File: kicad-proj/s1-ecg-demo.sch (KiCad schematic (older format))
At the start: 56 parts, among them J1 USB-C-16-Pin, J2 TC2030, J3 Battery Port, J4 Current Probe, J5 ECG_PAD_LA, J6 ECG_PAD_RA, J7 ECG_PAD_RL, U1 AD8233

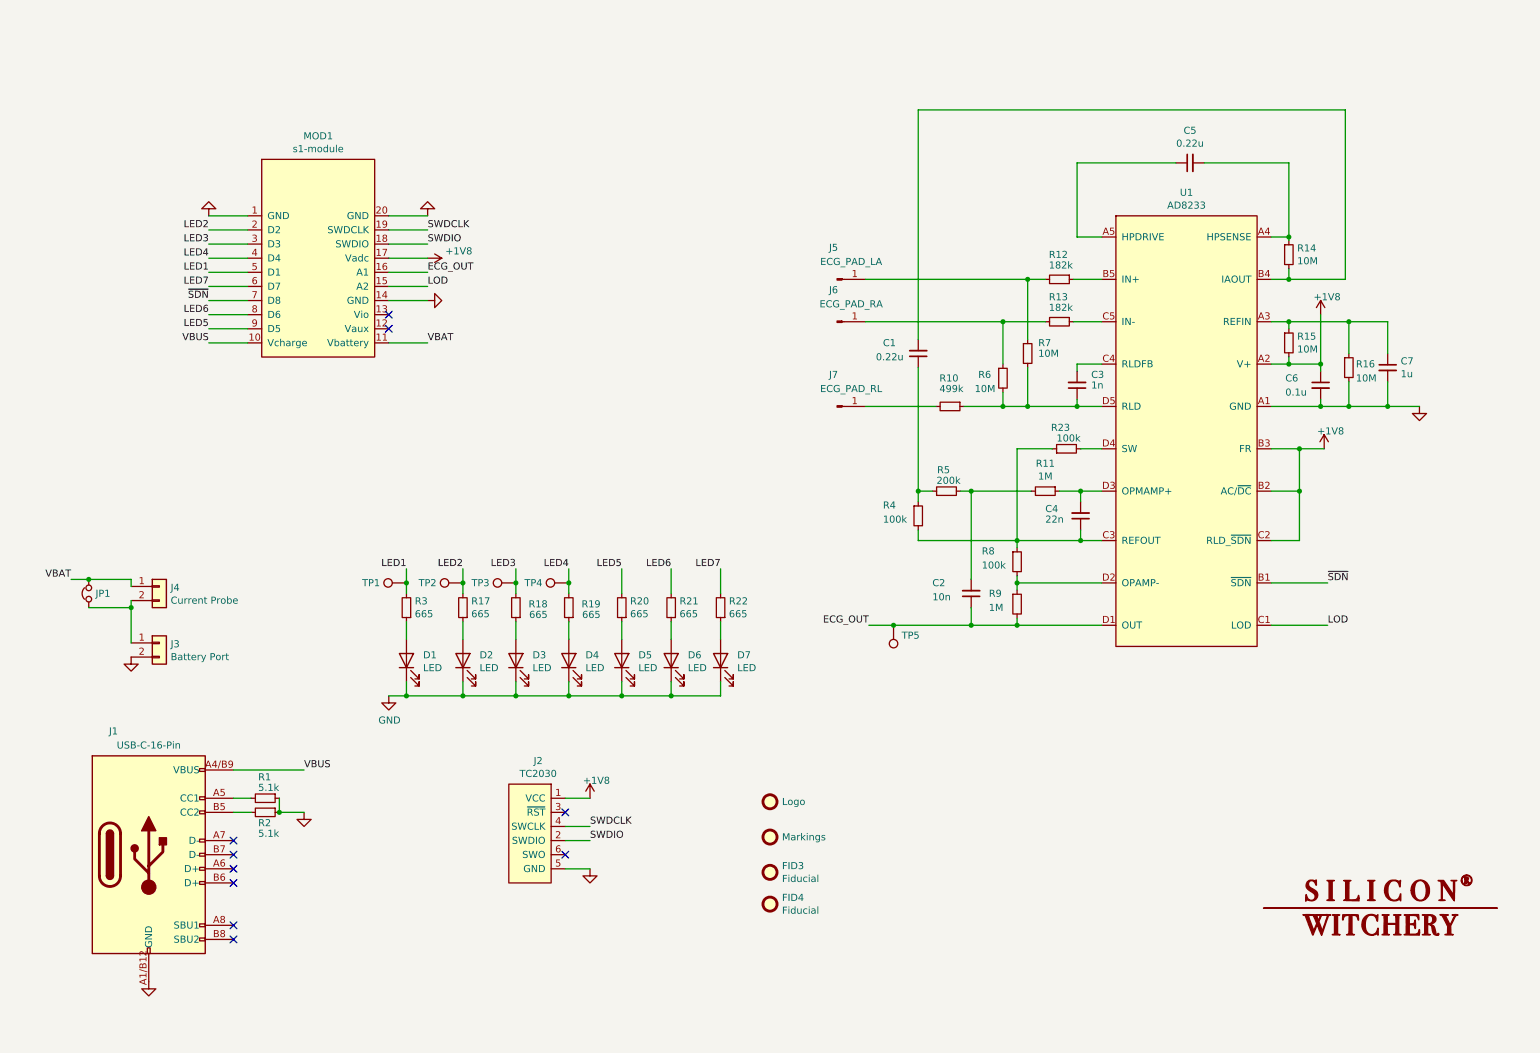
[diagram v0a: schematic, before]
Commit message: Layout complete, needs checking
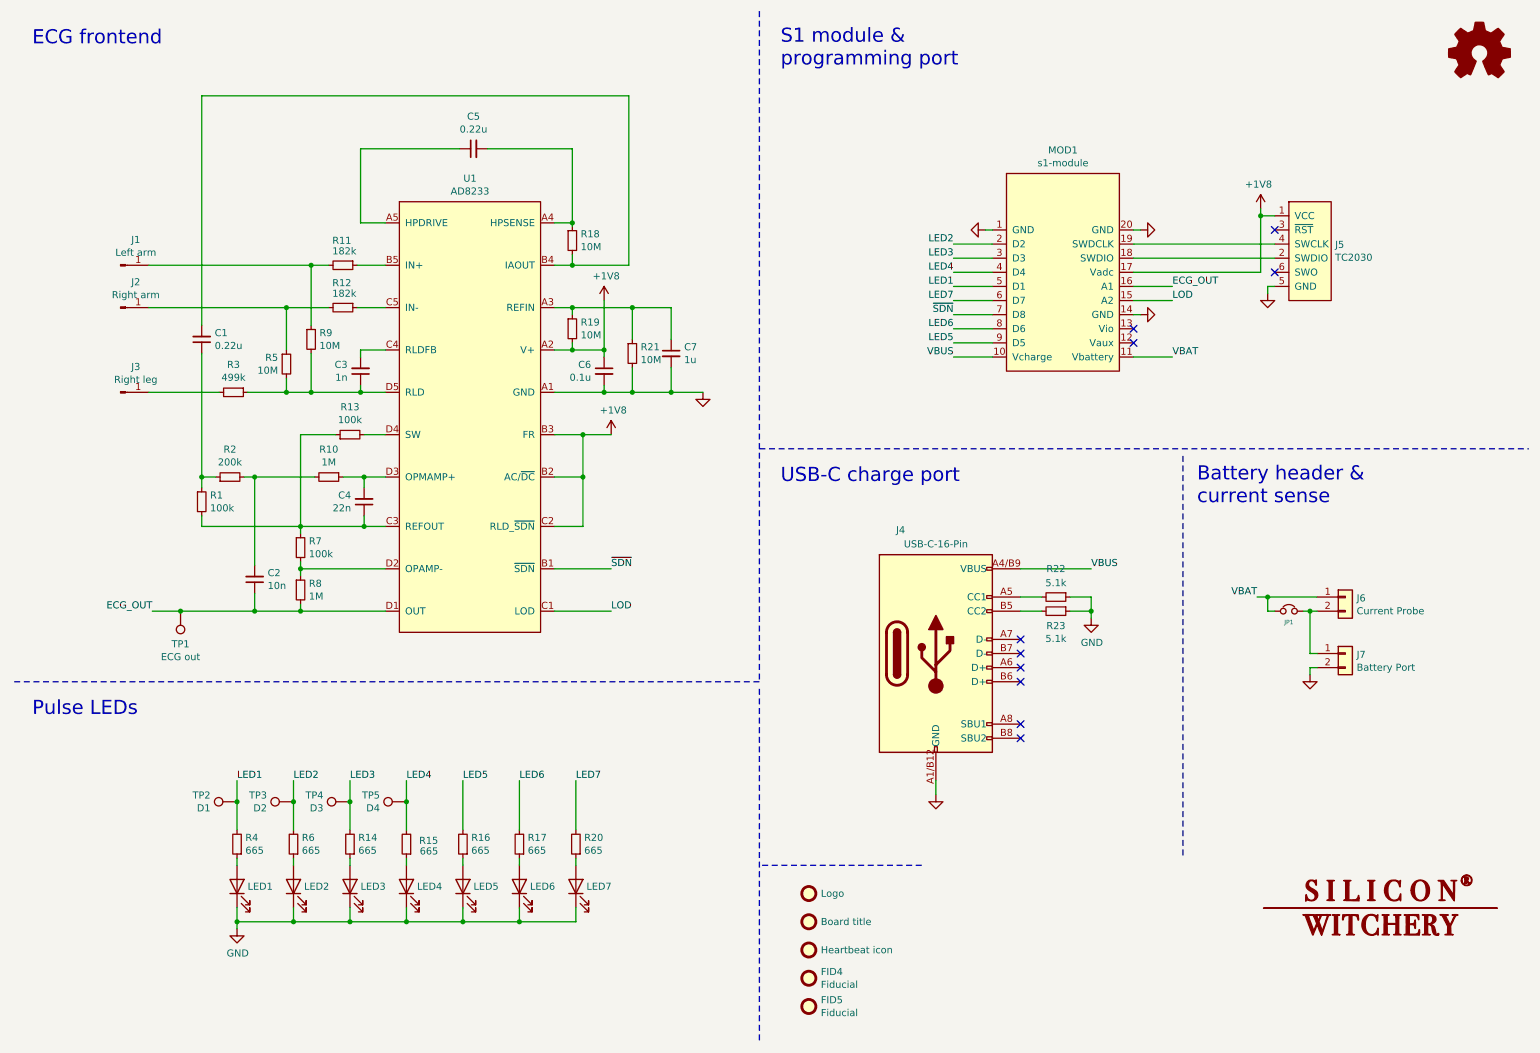
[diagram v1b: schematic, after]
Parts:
- added FID3: Heartbeat icon, s1-ecg-demo:heartbeat, symbol Mechanical:Fiducial
- FID1: footprint (none) -> s1-ecg-demo:sw-logo
- FID2: value Markings -> Board title; footprint (none) -> s1-ecg-demo:title
- J1: renamed from J5; value ECG_PAD_LA -> Left arm
- J2: renamed from J6; value ECG_PAD_RA -> Right arm
- J3: renamed from J7; value ECG_PAD_RL -> Right leg
- TP1: renamed from TP5; value Tp -> ECG out; footprint TestPoint:TestPoint_Pad_1.0x1.0mm -> TestPoint:TestPoint_Pad_D1.0mm
- TP2: renamed from TP1; value Tp -> D1; footprint TestPoint:TestPoint_Pad_1.0x1.0mm -> TestPoint:TestPoint_Pad_D1.0mm
- TP3: renamed from TP2; value Tp -> D2; footprint TestPoint:TestPoint_Pad_1.0x1.0mm -> TestPoint:TestPoint_Pad_D1.0mm
- TP4: renamed from TP3; value Tp -> D3; footprint TestPoint:TestPoint_Pad_1.0x1.0mm -> TestPoint:TestPoint_Pad_D1.0mm
- TP5: renamed from TP4; value Tp -> D4; footprint TestPoint:TestPoint_Pad_1.0x1.0mm -> TestPoint:TestPoint_Pad_D1.0mm
- renumbered FID3 to FID4, FID4 to FID5, J1 to J4, J2 to J5, J4 to J6, J3 to J7, D1 to LED1, D2 to LED2, D3 to LED3, D4 to LED4, D5 to LED5, D6 to LED6, D7 to LED7, R4 to R1, R11 to R10, R12 to R11, R13 to R12, R23 to R13, R18 to R14, R19 to R15, R20 to R16, R21 to R17, R14 to R18, R15 to R19, R5 to R2, R22 to R20, R16 to R21, R1 to R22, R2 to R23, R10 to R3, R3 to R4, R6 to R5, R17 to R6, R8 to R7, R9 to R8, R7 to R9
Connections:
- net SWDCLK: no longer names the net of J5.4 (SWCLK), MOD1.19 (SWDCLK)
- net SWDIO: no longer names the net of J5.2 (SWDIO), MOD1.18 (SWDIO)
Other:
- note added: "Battery header &\ncurrent sense"
- note added: "ECG frontend"
- note added: "Pulse LEDs"
- note added: "S1 module &\nprogramming port"
- note added: "USB-C charge port"
- moved on the sheet: C1, C2, C3, C4, C5, C6, C7, FID4, FID5, J1, J2, J3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

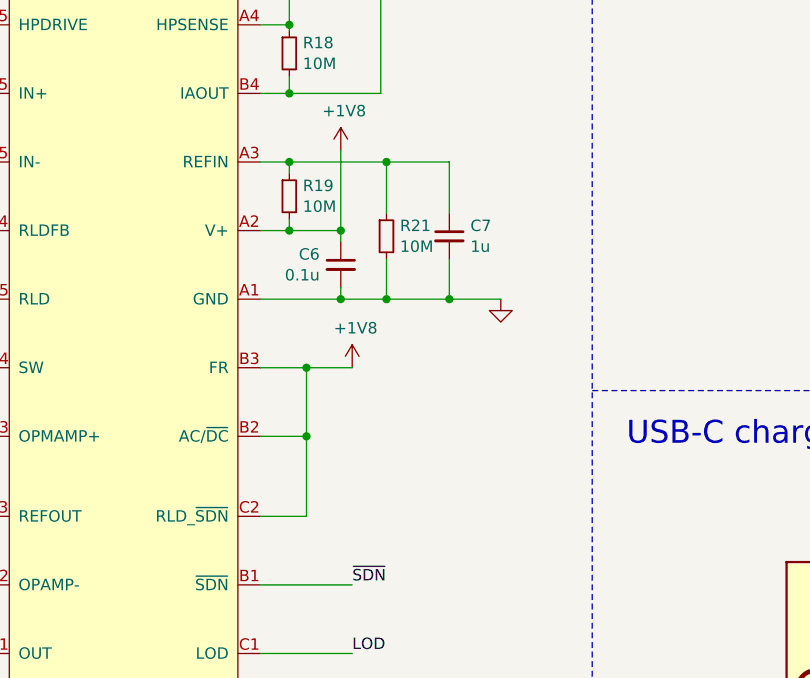
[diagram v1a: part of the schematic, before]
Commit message: Final check done
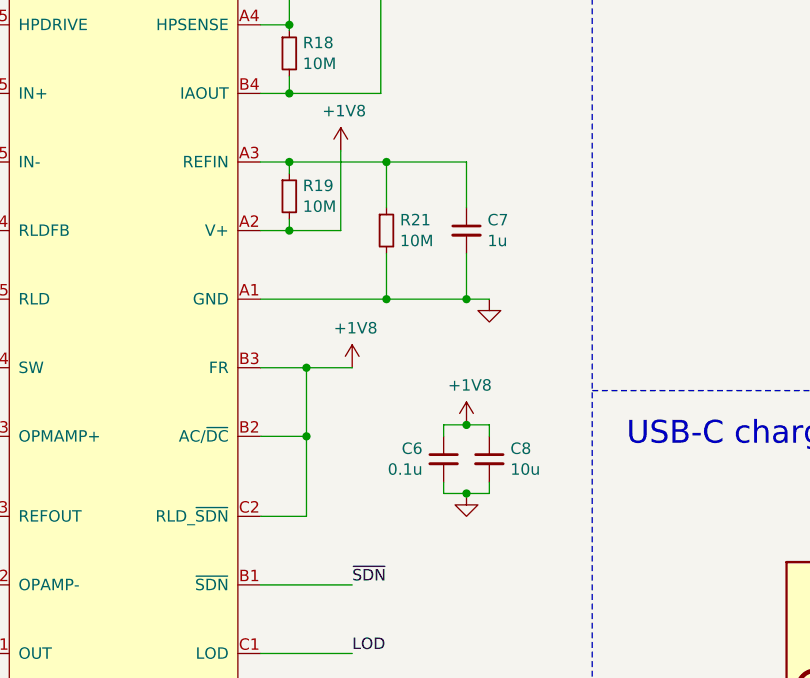
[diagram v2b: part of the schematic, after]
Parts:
- added C8: 10u, Capacitor_SMD:C_0402_1005Metric, symbol Device:C_Small
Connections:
- net +1V8: now also C8.1
- net GND: now also C8.2
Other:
- moved on the sheet: C6, C7, R21
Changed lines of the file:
@@
 L Device:C_Small C6
 U 1 1 6112DEAF
-P 4700 3050
-F 0 "C6" H 4608 3096 50  0000 R CNN
-F 1 "0.1u" H 4608 3005 50  0000 R CNN
-F 2 "Capacitor_SMD:C_0402_1005Metric" H 4700 3050 50  0001 C CNN
-F 3 "~" H 4700 3050 50  0001 C CNN
-	1    4700 3050
-	1    0    0    -1
-$EndComp
-$Comp
-L Device:C_Small C7
-U 1 1 6112EC74
-P 5175 2925
-F 0 "C7" H 5267 2971 50  0000 L CNN
-F 1 "1u" H 5267 2880 50  0000 L CNN
-F 2 "Capacitor_SMD:C_0402_1005Metric" H 5175 2925 50  0001 C CNN
-F 3 "~" H 5175 2925 50  0001 C CNN
-	1    5175 2925
+P 5150 3900
+F 0 "C6" H 5058 3946 50  0000 R CNN
+F 1 "0.1u" H 5058 3855 50  0000 R CNN
+F 2 "Capacitor_SMD:C_0402_1005Metric" H 5150 3900 50  0001 C CNN
+F 3 "~" H 5150 3900 50  0001 C CNN
+	1    5150 3900
 	1    0    0    -1
 $EndComp
@@
 	4875 2300 4475 2300
 Wire Wire Line
-	5175 2600 5175 2825
-Wire Wire Line
-	5175 3025 5175 3200
-Wire Wire Line
-	5175 3200 4900 3200
-Wire Wire Line
-	4700 3150 4700 3200
-Connection ~ 4700 3200
-Wire Wire Line
-	4700 3200 4350 3200
-Wire Wire Line
 	4350 2900 4475 2900
 Wire Wire Line
-	4700 2900 4700 2950
+	5150 3750 5150 3800
 Wire Wire Line
 	2225 4425 2225 3800
@@
 L Device:R_Small R21
 U 1 1 61162002
-P 4900 2925
-F 0 "R21" H 4959 2971 50  0000 L CNN
-F 1 "10M" H 4959 2880 50  0000 L CNN
-F 2 "Resistor_SMD:R_0201_0603Metric" H 4900 2925 50  0001 C CNN
-F 3 "~" H 4900 2925 50  0001 C CNN
-	1    4900 2925
-	1    0    0    -1
-$EndComp
-Wire Wire Line
-	4900 3025 4900 3200
-Connection ~ 4900 3200
-Wire Wire Line
-	4900 3200 4700 3200
-Wire Wire Line
-	4900 2825 4900 2600
-Connection ~ 4900 2600
-Wire Wire Line
-	4900 2600 5175 2600
+P 4900 2900
+F 0 "R21" H 4959 2946 50  0000 L CNN
+F 1 "10M" H 4959 2855 50  0000 L CNN
+F 2 "Resistor_SMD:R_0201_0603Metric" H 4900 2900 50  0001 C CNN
+F 3 "~" H 4900 2900 50  0001 C CNN
+	1    4900 2900
+	1    0    0    -1
+$EndComp
 Wire Wire Line
 	4350 3500 4550 3500
@@
 Wire Wire Line
 	7450 2950 7175 2950
-Wire Wire Line
-	5175 3200 5400 3200
-Connection ~ 5175 3200
 Text Label 1500 4750 2    50   ~ 0
 ECG_OUT
@@
 Wire Wire Line
 	4700 2900 4700 2550
-Connection ~ 4700 2900
 Text Label 8725 2950 0    50   ~ 0
 VBAT
@@
 $EndComp
 $Comp
-L power:GND #PWR09
+L power:GND #PWR011
 U 1 1 6127ADA9
 P 8500 2650
-F 0 "#PWR09" H 8500 2400 50  0001 C CNN
+F 0 "#PWR011" H 8500 2400 50  0001 C CNN
 F 1 "GND" H 8575 2700 50  0001 C CNN
 F 2 "" H 8500 2650 50  0001 C CNN
@@
 $EndComp
 $Comp
-L power:GND #PWR04
-U 1 1 612AC006
-P 5400 3200
-F 0 "#PWR04" H 5400 2950 50  0001 C CNN
-F 1 "GND" H 5475 3250 50  0001 C CNN
-F 2 "" H 5400 3200 50  0001 C CNN
-F 3 "" H 5400 3200 50  0001 C CNN
-	1    5400 3200
-	1    0    0    -1
-$EndComp
-$Comp
-L power:GND #PWR06
+L power:GND #PWR08
 U 1 1 612FCD59
 P 7400 2050
-F 0 "#PWR06" H 7400 1800 50  0001 C CNN
+F 0 "#PWR08" H 7400 1800 50  0001 C CNN
 F 1 "GND" H 7475 2100 50  0001 C CNN
 F 2 "" H 7400 2050 50  0001 C CNN
@@
 $EndComp
 $Comp
-L power:GND #PWR05
+L power:GND #PWR07
 U 1 1 61355C6C
 P 7050 6050
-F 0 "#PWR05" H 7050 5800 50  0001 C CNN
+F 0 "#PWR07" H 7050 5800 50  0001 C CNN
 F 1 "GND" H 7125 6100 50  0001 C CNN
 F 2 "" H 7050 6050 50  0001 C CNN
@@
 $EndComp
 $Comp
-L power:GND #PWR08
+L power:GND #PWR010
 U 1 1 61359CD0
 P 8500 2050
-F 0 "#PWR08" H 8500 1800 50  0001 C CNN
+F 0 "#PWR010" H 8500 1800 50  0001 C CNN
 F 1 "GND" H 8575 2100 50  0001 C CNN
 F 2 "" H 8500 2050 50  0001 C CNN
@@
 $EndComp
 $Comp
-L power:GND #PWR012
+L power:GND #PWR014
 U 1 1 6135CB63
 P 9700 5200
-F 0 "#PWR012" H 9700 4950 50  0001 C CNN
+F 0 "#PWR014" H 9700 4950 50  0001 C CNN
 F 1 "GND" H 9775 5250 50  0001 C CNN
 F 2 "" H 9700 5200 50  0001 C CNN
@@
 $EndComp
 $Comp
-L power:+1V8 #PWR010
+L power:+1V8 #PWR012
 U 1 1 6126BDB5
 P 9350 1900
-F 0 "#PWR010" H 9350 1750 50  0001 C CNN
+F 0 "#PWR012" H 9350 1750 50  0001 C CNN
 F 1 "+1V8" H 9365 2073 50  0000 C CNN
 F 2 "" H 9350 1900 50  0001 C CNN
@@
 Connection ~ 9350 1950
 $Comp
-L power:GND #PWR011
+L power:GND #PWR013
 U 1 1 613CFB69
 P 9400 2500
-F 0 "#PWR011" H 9400 2250 50  0001 C CNN
+F 0 "#PWR013" H 9400 2250 50  0001 C CNN
 F 1 "GND" H 9475 2550 50  0001 C CNN
 F 2 "" H 9400 2500 50  0001 C CNN
@@
 	8150 4750 8000 4750
 $Comp
-L power:GND #PWR07
+L power:GND #PWR09
 U 1 1 61766FFE
 P 8150 4800
-F 0 "#PWR07" H 8150 4550 50  0001 C CNN
+F 0 "#PWR09" H 8150 4550 50  0001 C CNN
 F 1 "GND" H 8155 4627 50  0000 C CNN
 F 2 "" H 8150 4800 50  0001 C CNN
@@
 	1    0    0    -1
 $EndComp
+$Comp
+L Device:C_Small C7
+U 1 1 6112EC74
+P 5250 2900
+F 0 "C7" H 5342 2946 50  0000 L CNN
+F 1 "1u" H 5342 2855 50  0000 L CNN
+F 2 "Capacitor_SMD:C_0402_1005Metric" H 5250 2900 50  0001 C CNN
+F 3 "~" H 5250 2900 50  0001 C CNN
+	1    5250 2900
+	1    0    0    -1
+$EndComp
+$Comp
+L power:GND #PWR06
+U 1 1 612AC006
+P 5350 3200
+F 0 "#PWR06" H 5350 2950 50  0001 C CNN
+F 1 "GND" H 5425 3250 50  0001 C CNN
+F 2 "" H 5350 3200 50  0001 C CNN
+F 3 "" H 5350 3200 50  0001 C CNN
+	1    5350 3200
+	1    0    0    -1
+$EndComp
+Wire Wire Line
+	5250 3200 5250 3000
+Connection ~ 5250 3200
+Wire Wire Line
+	5250 3200 5350 3200
+Wire Wire Line
+	4900 2600 4900 2800
+Connection ~ 4900 3200
+Wire Wire Line
+	4900 3200 5250 3200
+$Comp
+L Device:C_Small C8
+U 1 1 6123F165
+P 5350 3900
+F 0 "C8" H 5442 3946 50  0000 L CNN
+F 1 "10u" H 5442 3855 50  0000 L CNN
+F 2 "Capacitor_SMD:C_0402_1005Metric" H 5350 3900 50  0001 C CNN
+F 3 "~" H 5350 3900 50  0001 C CNN
+	1    5350 3900
+	1    0    0    -1
+$EndComp
+Wire Wire Line
+	5250 2800 5250 2600
+Wire Wire Line
+	5250 2600 4900 2600
+Connection ~ 4900 2600
+Wire Wire Line
+	5350 3800 5350 3750
+Wire Wire Line
+	4900 3000 4900 3200
+Wire Wire Line
+	4350 3200 4900 3200
+$Comp
+L power:+1V8 #PWR04
+U 1 1 612AFAB8
+P 5250 3750
+F 0 "#PWR04" H 5250 3600 50  0001 C CNN
+F 1 "+1V8" H 5265 3923 50  0000 C CNN
+F 2 "" H 5250 3750 50  0001 C CNN
+F 3 "" H 5250 3750 50  0001 C CNN
+	1    5250 3750
+	1    0    0    -1
+$EndComp
+$Comp
+L power:GND #PWR05
+U 1 1 612AFCE8
+P 5250 4050
+F 0 "#PWR05" H 5250 3800 50  0001 C CNN
+F 1 "GND" H 5325 4100 50  0001 C CNN
+F 2 "" H 5250 4050 50  0001 C CNN
+F 3 "" H 5250 4050 50  0001 C CNN
+	1    5250 4050
+	1    0    0    -1
+$EndComp
+Wire Wire Line
+	5350 3750 5250 3750
+Connection ~ 5250 3750
+Wire Wire Line
+	5250 3750 5150 3750
+Wire Wire Line
+	5250 4050 5150 4050
+Wire Wire Line
+	5150 4050 5150 4000
+Wire Wire Line
+	5250 4050 5350 4050
+Wire Wire Line
+	5350 4050 5350 4000
+Connection ~ 5250 4050
 $EndSCHEMATC
